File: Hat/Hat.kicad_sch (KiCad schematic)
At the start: 86 parts, among them J1 Conn_01x01_Pin, J2 Conn_01x12_Pin, J3 Conn_01x12_Pin, J4 Conn_01x06_Pin, Q1 BC547, Q10 BC547, Q3 BC547, Q4 BC547, Q6 BC547, Q7 BC547, Q8 BC547, Q8 BC557, SW1 SW_Push, SW2 SW_SPDT, U1 TL074, U13 Aux_flush, U5 4066

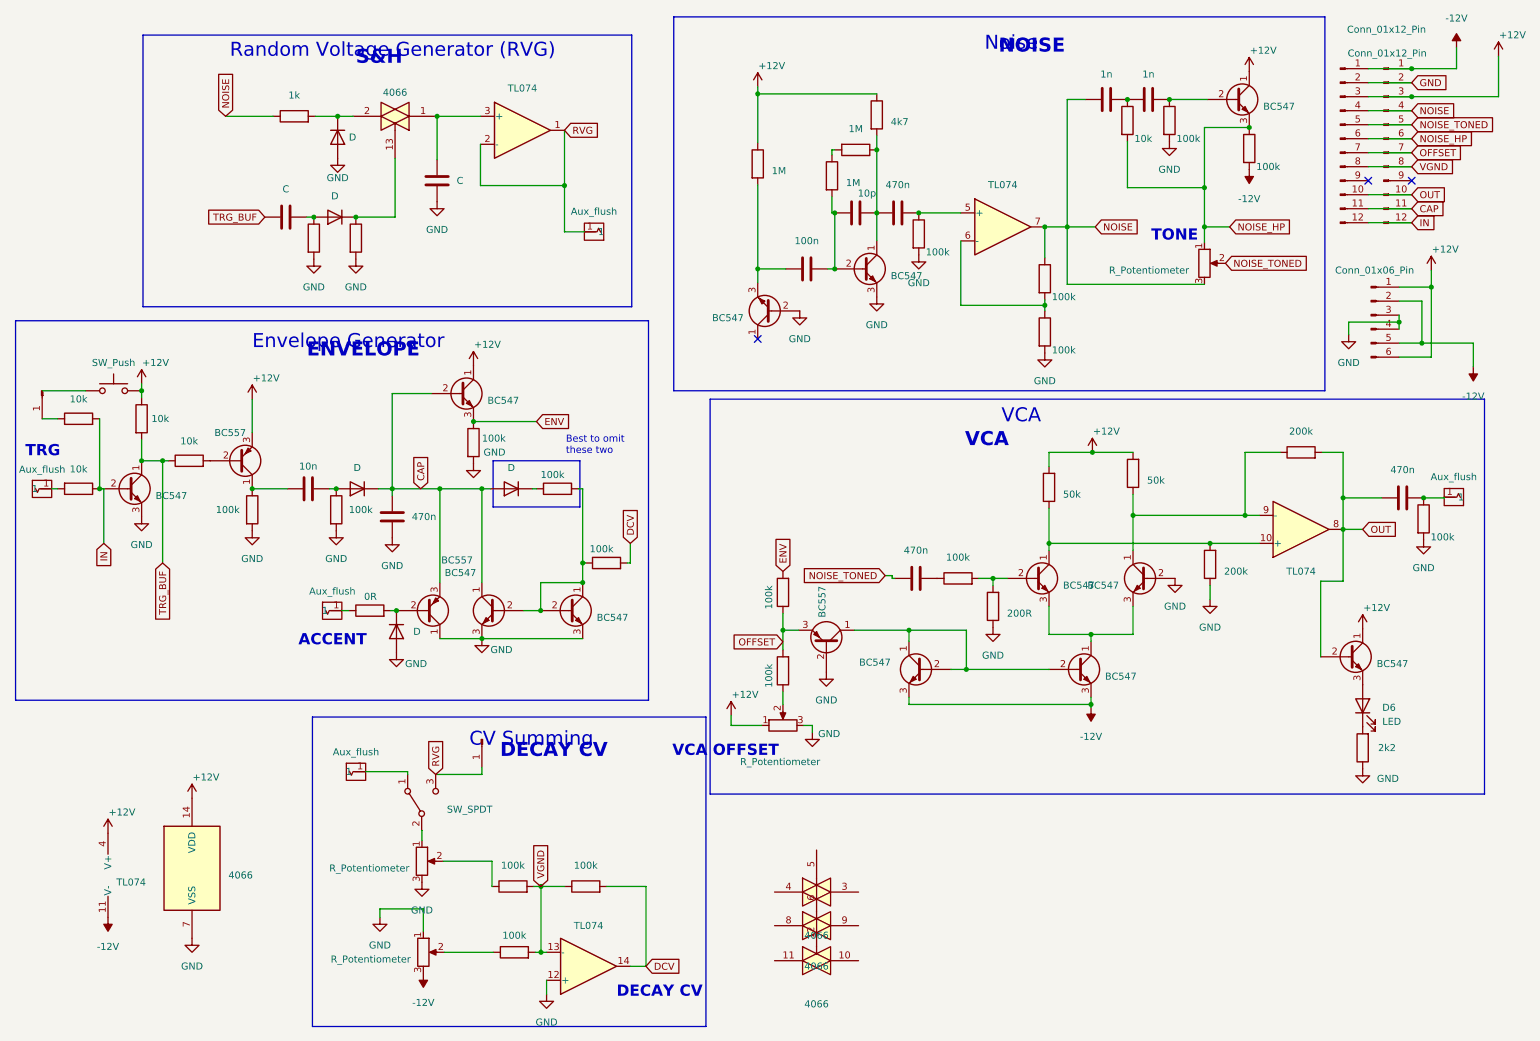
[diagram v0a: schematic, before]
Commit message: Add files via upload
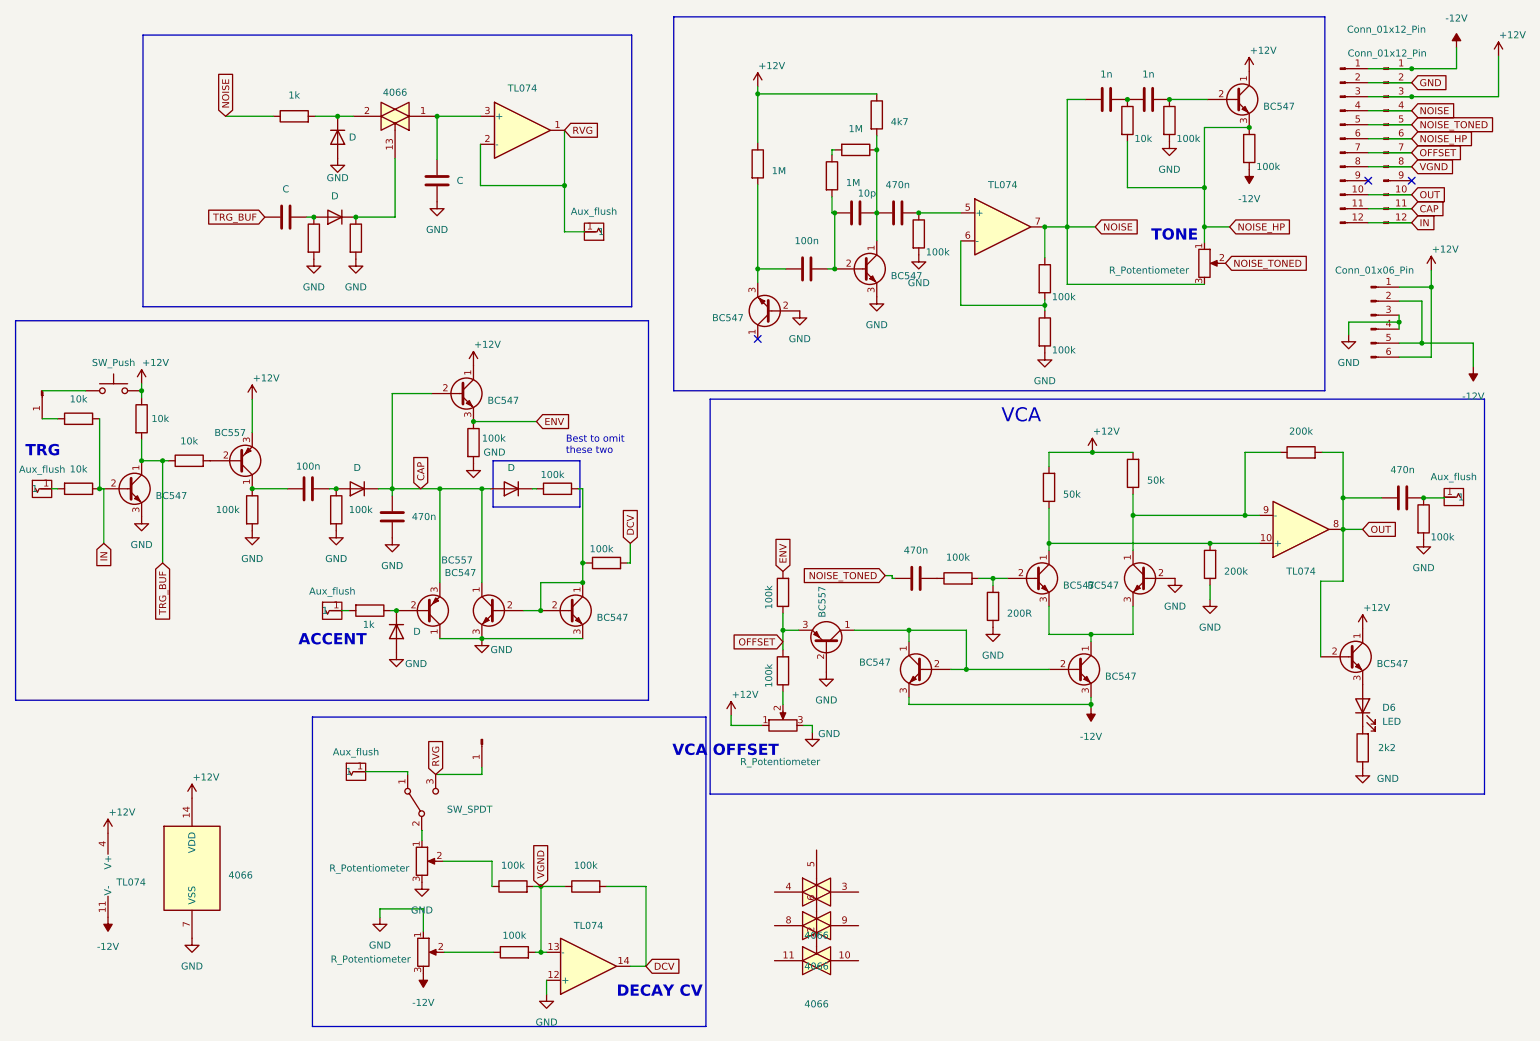
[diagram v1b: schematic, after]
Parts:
- C3: value 10n -> 100n
- R42: value 0R -> 1k
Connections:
- net at D8.1 (K), Q8.2 (B): now also R42.1; no longer R42.2
- net at U13.1: now also R42.2; no longer R42.1
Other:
- note removed: "CV Summing"
- note removed: "ENVELOPE"
- note removed: "Envelope Generator"
- note removed: "NOISE"
- note removed: "Noise"
- note removed: "Random Voltage Generator (RVG)"
- note removed: "S&H"
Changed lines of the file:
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@@
     (fill (type none))
-  )
-  (text "S&H\n" (at 74.93 22.606 0)
-    (effects (font (size 2.54 2.54) (thickness 0.508) bold) (justify left bottom))
-  )
-  (text "Noise" (at 188.976 20.066 0)
-    (effects (font (size 2.54 2.54)) (justify left bottom) hide)
-  )
-  (text "ENVELOPE\n" (at 66.04 75.692 0)
-    (effects (font (size 2.54 2.54) (thickness 0.508) bold) (justify left bottom))
-  )
-  (text "CV Summing\n" (at 95.504 146.304 0)
-    (effects (font (size 2.54 2.54)) (justify left bottom) hide)
   )
   (text "TRG" (at 14.986 93.726 0)
@@
     (effects (font (size 2.54 2.54)) (justify left bottom) hide)
   )
-  (text "Envelope Generator\n" (at 56.134 74.168 0)
-    (effects (font (size 2.54 2.54)) (justify left bottom) hide)
-  )
-  (text "VCA\n" (at 185.42 91.948 0)
-    (effects (font (size 2.54 2.54) (thickness 0.508) bold) (justify left bottom))
-  )
   (text "TONE\n" (at 219.202 54.61 0)
     (effects (font (size 2.032 2.032) (thickness 1.524) bold) (justify left bottom) hide)
@@
     (effects (font (size 2.032 2.032) (thickness 1.524) bold) (justify left bottom) hide)
   )
-  (text "Random Voltage Generator (RVG)" (at 52.07 21.336 0)
-    (effects (font (size 2.54 2.54)) (justify left bottom) hide)
-  )
-  (text "DECAY CV\n" (at 101.092 148.336 0)
-    (effects (font (size 2.54 2.54) (thickness 0.508) bold) (justify left bottom))
-  )
   (text "DECAY CV\n" (at 122.2248 191.77 0)
     (effects (font (size 2.032 2.032) (thickness 1.524) bold) (justify left bottom) hide)
-  )
-  (text "NOISE" (at 191.516 20.574 0)
-    (effects (font (size 2.54 2.54) (thickness 0.508) bold) (justify left bottom))
   )
   (text "ACCENT\n" (at 64.516 128.016 0)
@@
       (effects (font (size 1.27 1.27)) hide)
     )
-    (property "Value" "10n" (at 66.294 95.25 90)
+    (property "Value" "100n" (at 66.294 95.25 90)
       (effects (font (size 1.27 1.27)))
     )
@@
     )
   )
-  (symbol (lib_id "Device:R") (at 77.47 121.412 90) (unit 1)
+  (symbol (lib_id "Device:R") (at 77.47 121.412 270) (unit 1)
     (in_bom yes) (on_board yes) (dnp no)
-    (property "Reference" "R42" (at 76.1999 118.872 0)
-      (effects (font (size 1.27 1.27)) (justify left) hide)
-    )
-    (property "Value" "0R" (at 78.7399 118.872 90)
+    (property "Reference" "R42" (at 78.7401 123.952 0)
+      (effects (font (size 1.27 1.27)) (justify left) hide)
+    )
+    (property "Value" "1k" (at 76.2001 123.952 90)
       (effects (font (size 1.27 1.27)) (justify left))
     )
-    (property "Footprint" "Resistor_THT:R_Axial_DIN0204_L3.6mm_D1.6mm_P7.62mm_Horizontal" (at 77.47 123.19 90)
-      (effects (font (size 1.27 1.27)) hide)
-    )
+    (property "Footprint" "Resistor_THT:R_Axial_DIN0204_L3.6mm_D1.6mm_P7.62mm_Horizontal" (at 77.47 119.634 90)
+      (effects (font (size 1.27 1.27)) hide)
+    )
